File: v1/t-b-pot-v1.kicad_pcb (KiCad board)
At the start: 2 copper layers, 20.6 x 31 mm, 9 parts

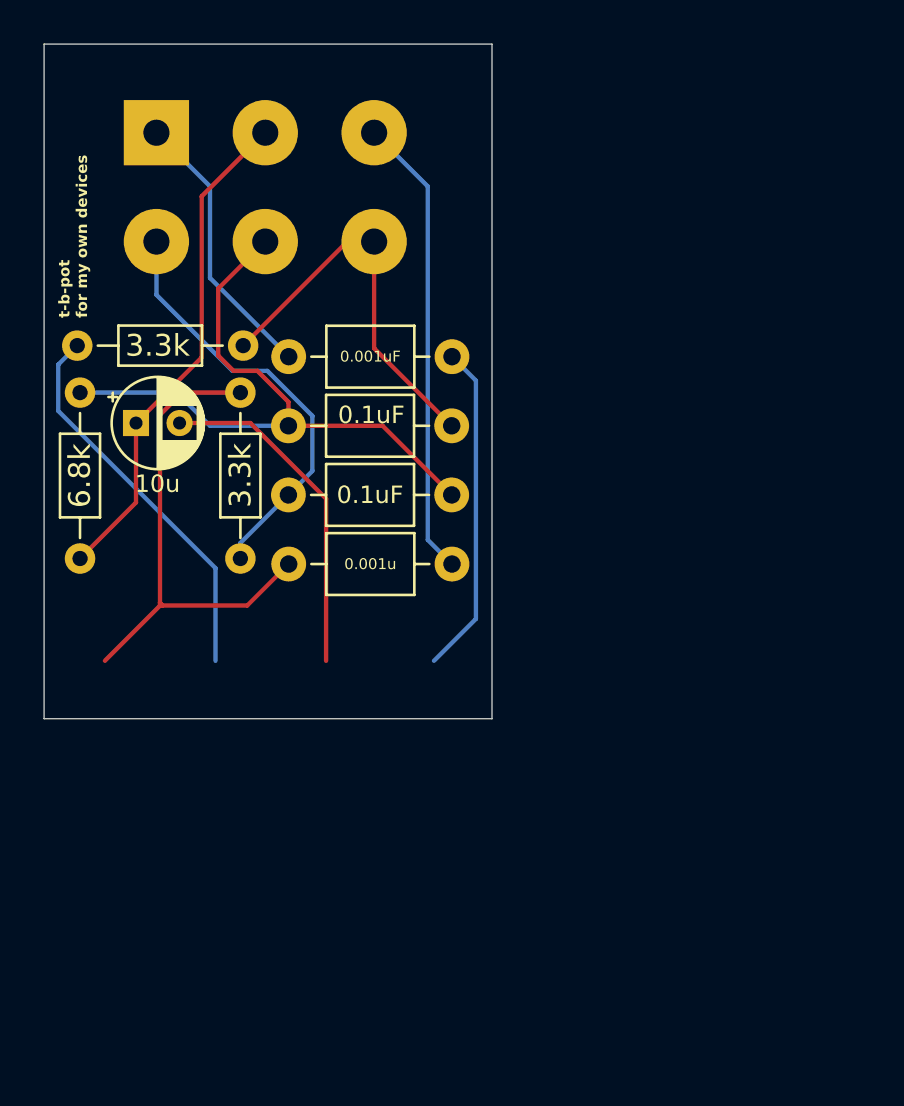
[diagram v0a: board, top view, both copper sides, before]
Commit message: updates circuit
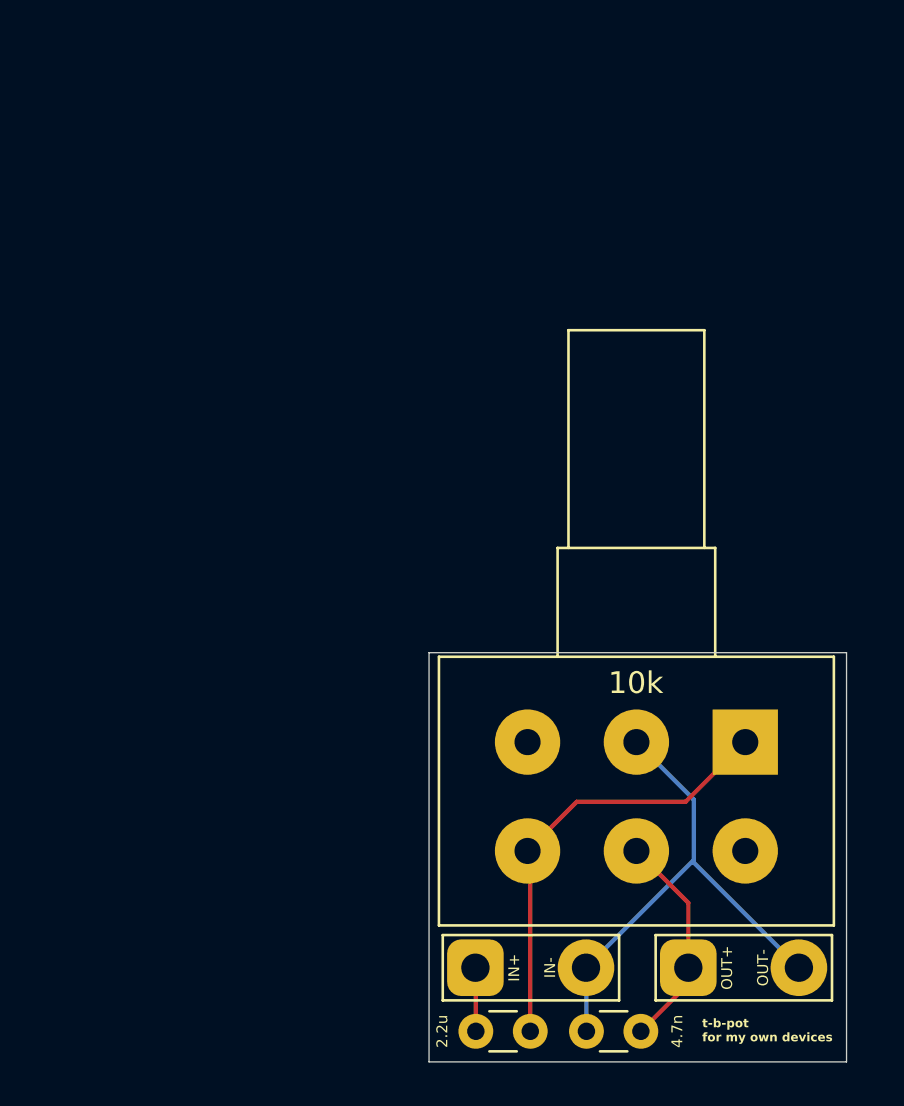
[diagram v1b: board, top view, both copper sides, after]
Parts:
- removed C3: 10u, Capacitor_THT:CP_Radial_D4.0mm_P2.00mm
- removed C4: 0.001u, Capacitor_THT:C_Axial_L3.8mm_D2.6mm_P7.50mm_Horizontal
- removed C5: 0.001uF, Capacitor_THT:C_Axial_L3.8mm_D2.6mm_P7.50mm_Horizontal
- removed R1, R2: 3.3k, Resistor_THT:R_Axial_DIN0204_L3.6mm_D1.6mm_P7.62mm_Horizontal
- removed R3: 6.8k, Resistor_THT:R_Axial_DIN0204_L3.6mm_D1.6mm_P7.62mm_Horizontal
- added I1: 1, TestPoint:TestPoint_2Pads_Pitch5.08mm_Drill1.3mm, F.Cu at (159.1, 118.1)
- added V2: VSIN, TestPoint:TestPoint_2Pads_Pitch5.08mm_Drill1.3mm, F.Cu at (149.4, 118.1)
- C1: value 0.1uF -> 2.2u; footprint Capacitor_THT:C_Axial_L3.8mm_D2.6mm_P7.50mm_Horizontal -> Capacitor_THT:C_Disc_D3.0mm_W1.6mm_P2.50mm
- C2: value 0.1uF -> 4.7n; footprint Capacitor_THT:C_Axial_L3.8mm_D2.6mm_P7.50mm_Horizontal -> Capacitor_THT:C_Disc_D3.0mm_W1.6mm_P2.50mm
- RV1: value R_Potentiometer_Dual -> 10k; moved to F.Cu
- moved RV1 38.9 mm to (161.7, 107.7)
- moved C2 32.2 mm to (157.0, 121.0), turned to 180 degrees
- moved C1 26.1 mm to (149.4, 121.0)
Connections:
- C2 pad 1: Net-(C1-Pad2) -> Net-(C2-Pad1)
- C2 pad 2: Net-(C2-Pad2) -> GND
- RV1 pad 1: Net-(C5-Pad2) -> Net-(C1-Pad2)
- RV1 pad 2: Net-(C3-Pad1) -> GND
- RV1 pad 3: Net-(C4-Pad1) -> unconnected-(RV1-Pad3)
- RV1 pad 4: Net-(C1-Pad1) -> unconnected-(RV1-Pad4)
- RV1 pad 5: Net-(C1-Pad2) -> Net-(C2-Pad1)
- RV1 pad 6: Net-(C2-Pad2) -> Net-(C1-Pad2)
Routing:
- net Net-(C4-Pad2): track 23.2 -> 0.00 mm
- net Net-(C3-Pad1): track 23.1 -> 0.00 mm
- net Net-(C4-Pad1): track 21.3 -> 0.00 mm
- net Net-(C2-Pad2): track 17.9 -> 0.00 mm
- net Net-(C1-Pad1): track 19.8 -> 2.93 mm
- net Net-(C3-Pad2): track 15.6 -> 0.00 mm
- net Net-(C5-Pad2): track 12.8 -> 0.00 mm
- net Net-(C2-Pad1): track 0.00 -> 10.2 mm
- net Net-(C1-Pad2): track 30.4 -> 20.4 mm
- net GND: track 33.1 -> 23.4 mm
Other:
- board size 20.6 x 31 mm -> 19.2 x 18.8 mm
